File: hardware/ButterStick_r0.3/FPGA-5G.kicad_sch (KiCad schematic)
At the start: 1 part, among them U4 ECP5UM5G_85_CABGA381

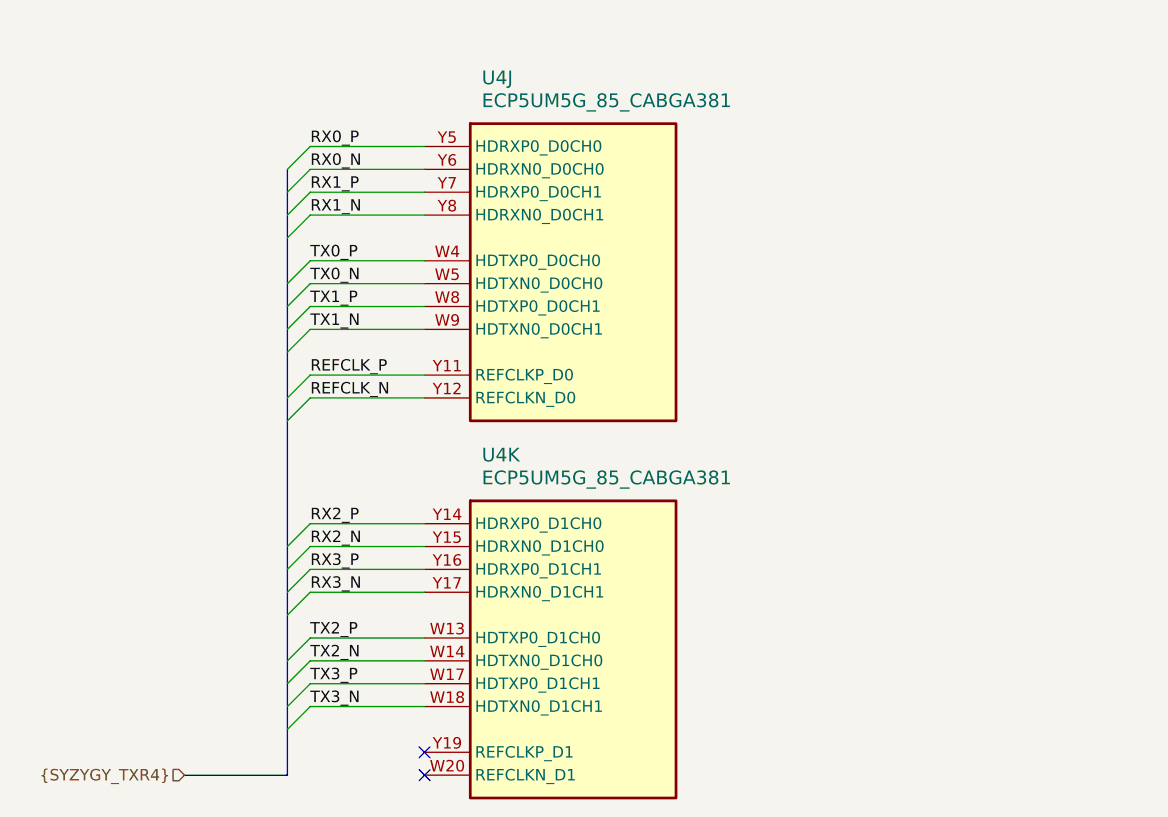
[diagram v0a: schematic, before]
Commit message: hw.r0d3: complete first pass of routing
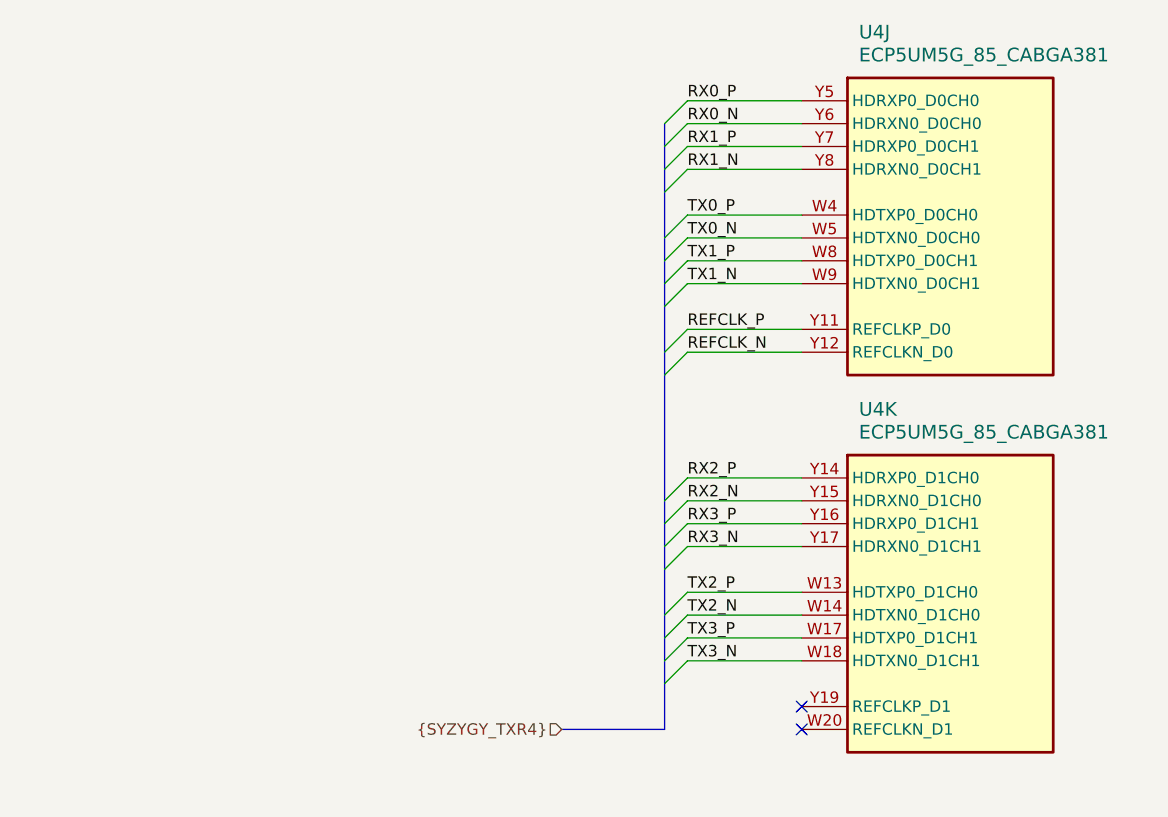
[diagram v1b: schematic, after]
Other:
- moved on the sheet: U4J, U4K
